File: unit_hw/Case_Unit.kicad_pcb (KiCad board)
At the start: 2 copper layers, 16.1 x 33.6 mm, 15 parts, among them J1 Conn_01x04, J3 RJ45, J4 Conn_01x03, U1 SPX3819M5-L-3-3, U2 STM32G030F6Px, U3 MAX487E

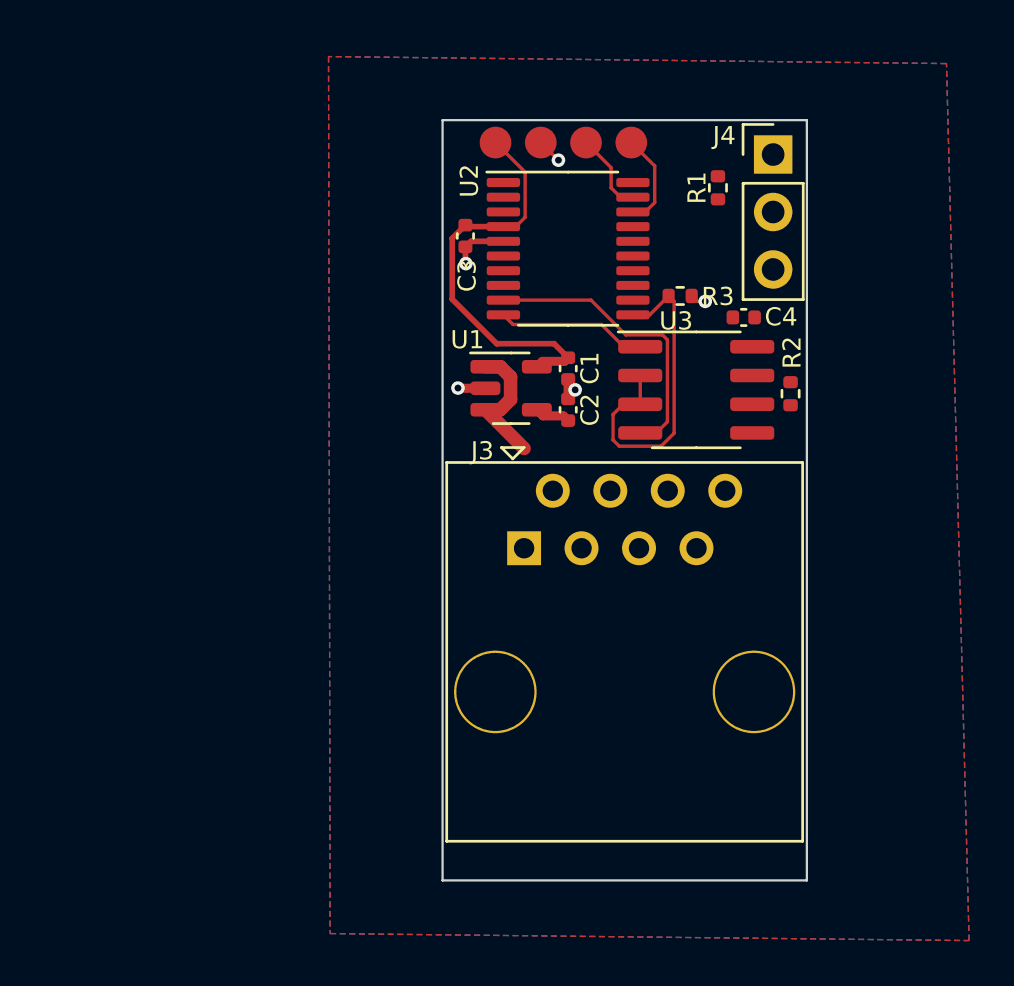
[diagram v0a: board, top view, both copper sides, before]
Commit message: Submit for fab (Rev. 2 unit)
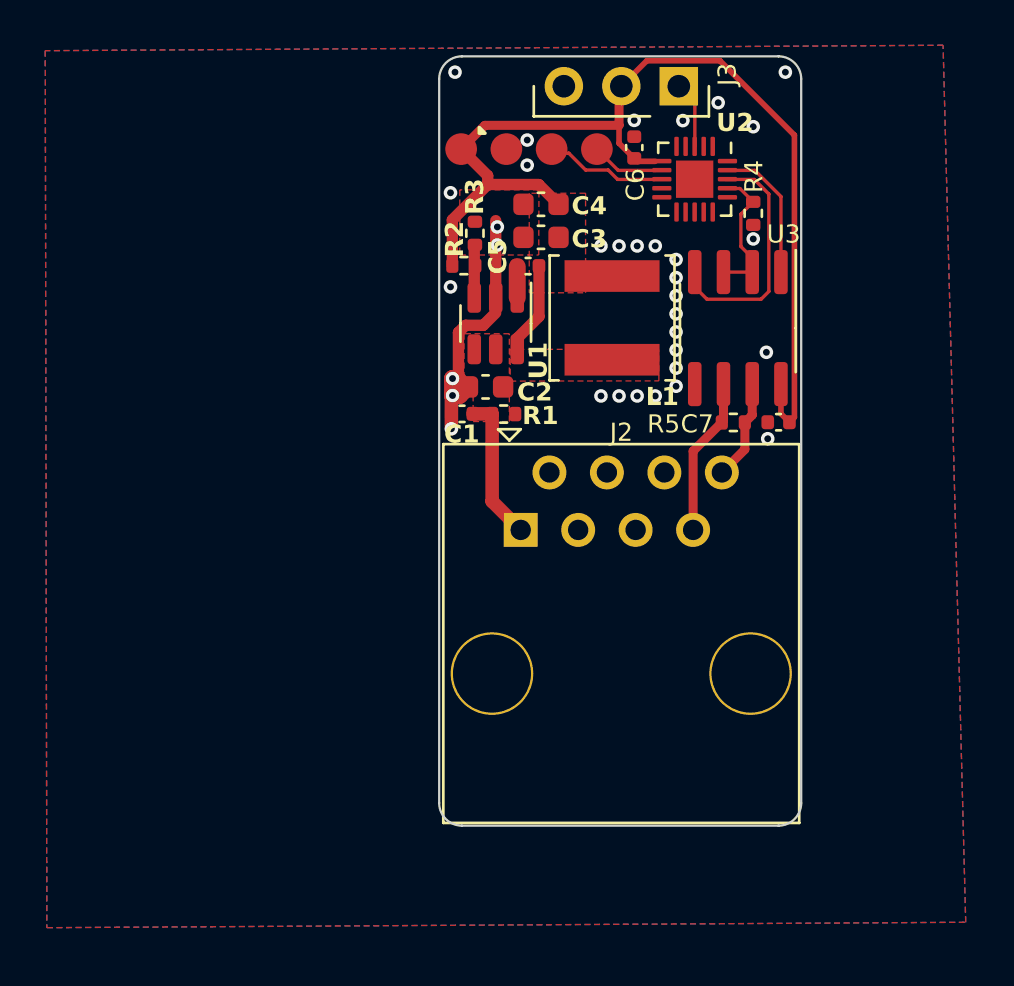
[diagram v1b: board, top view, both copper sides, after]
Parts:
- added C3: 22u, Capacitor_SMD:C_0603_1608Metric, F.Cu at (69.5, 40.0)
- added C4: 22u, Capacitor_SMD:C_0603_1608Metric, F.Cu at (69.5, 38.5)
- added C5: 100n, Capacitor_SMD:C_0402_1005Metric, F.Cu at (68.9, 41.3)
- added L1: 10u, Inductor_SMD:L_Changjiang_FNR5030S, F.Cu at (72.6, 43.6)
- added R2: 100k, Resistor_SMD:R_0402_1005Metric, F.Cu at (66.1, 41.2)
- added R3: 13k, Resistor_SMD:R_0402_1005Metric, F.Cu at (66.6, 39.8)
- C1: value 4.7u -> 100n
- C2: value 10n -> 22u; footprint Capacitor_SMD:C_0402_1005Metric -> Capacitor_SMD:C_0603_1608Metric
- R1: value 4.7k -> 1
- U1: value SPX3819M5-L-3-3 -> MT2492; footprint Package_TO_SOT_SMD:SOT-23-5 -> Package_TO_SOT_SMD:SOT-23-6
- U2: value STM32G030F6Px -> PY32F003F18U6; footprint Package_SO:TSSOP-20_4.4x6.5mm_P0.65mm -> Package_DFN_QFN:QFN-20-1EP_3x3mm_P0.4mm_EP1.65x1.65mm
- moved R1 13.8 mm to (67.8, 47.8), turned to 0 degrees
- moved C6 8.42 mm to (73.6, 36.0), turned to 90 degrees
- moved U2 6.38 mm to (76.3, 37.4), turned to -90 degrees
- moved J3 5.15 mm to (75.6, 33.3), turned to -90 degrees
- moved C1 5.10 mm to (66.0, 47.8), turned to 180 degrees
- moved C7 4.88 mm to (80.0, 48.2), turned to 180 degrees
- moved R4 4.87 mm to (78.9, 38.9), turned to -90 degrees
- moved C2 3.79 mm to (67.0, 46.6), turned to 180 degrees
- moved U3 3.29 mm to (78.2, 44.0), turned to -90 degrees
- moved U1 2.94 mm to (67.5, 43.8), turned to -90 degrees
- moved R5 2.83 mm to (78.0, 48.2), turned to 180 degrees
- moved J1 1.55 mm to (69.0, 36.1)
- moved J2 0.82 mm to (68.6, 52.9)
- moved G*** 0.53 mm to (70.8, 41.6)
- moved G*** 0.53 mm to (70.6, 36.6)
- renumbered C3 to C6, C4 to C7, J3 to J2, J4 to J3, R3 to R4, R2 to R5
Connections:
- C1 pad 1: +3V3 -> VIN
- C2 pad 1: Net-(U1-BP) -> Net-(U1-EN)
- C6 pad 1: +3V3 -> +5V
- J1 pad 1: +3V3 -> +5V
- J2 pad 1: +5V -> VIN
- J2 pad 3: unconnected-(J3-Pad3) -> GND
- J2 pad 4: unconnected-(J3-Pad4) -> GND
- J2 pad 5: unconnected-(J3-Pad5) -> GND
- J2 pad 6: unconnected-(J3-Pad6) -> GND
- R1 pad 1: +5V -> VIN
- R1 pad 2: /SERVO_OUT -> Net-(U1-EN)
- U1 pad 1: +5V -> Net-(U1-BS)
- U1 pad 3: +5V -> Net-(U1-FB)
- U1 pad 4: Net-(U1-BP) -> Net-(U1-EN)
- U1 pad 5: +3V3 -> Net-(U1-EN)
- U2 pad 10: /UART_RX -> unconnected-(U2-PB6-Pad10)
- U2 pad 11: /MAX487_DE -> unconnected-(U2-PB7-Pad11)
- U2 pad 14: /SERVO_OUT -> unconnected-(U2-PF1-Pad14)
- U2 pad 17: unconnected-(U2-PA12/PA10-Pad17) -> /MAX487_DE
- U2 pad 18: /SWDIO -> /UART_TX
- U2 pad 19: /SWCLK -> /UART_RX
- U2 pad 3: unconnected-(U2-PC15-Pad3) -> /SERVO_OUT
- U2 pad 4: +3V3 -> GND
- U2 pad 5: GND -> unconnected-(U2-PA12-Pad5)
- U2 pad 6: unconnected-(U2-NRST-Pad6) -> +5V
- U2 pad 7: unconnected-(U2-PA0-Pad7) -> /SWDIO
- U2 pad 8: unconnected-(U2-PA1-Pad8) -> /SWCLK
- U2 pad 9: /UART_TX -> unconnected-(U2-PB5-Pad9)
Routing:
- net +5V: track 6.01 -> 45.8 mm
- net +3V3: track 17.9 -> 0.00 mm
- net /MAX487_DE: track 14.9 -> 6.28 mm
- net /RS422+: track 0.00 -> 7.00 mm
- net VIN: track 0.00 -> 6.48 mm
- net GND: track 6.40 -> 11.7 mm, vias 5 -> 34
- net /RS422-: track 0.00 -> 4.46 mm
- net Net-(U1-SW): track 0.00 -> 4.08 mm
- net /SERVO_OUT: track 0.00 -> 2.79 mm
- net Net-(U1-FB): track 0.00 -> 2.35 mm
- net /UART_TX: track 13.0 -> 10.8 mm
- net Net-(U1-BP): track 1.58 -> 0.00 mm
- net /SWCLK: track 3.60 -> 5.14 mm
- net Net-(U1-BS): track 0.00 -> 1.38 mm
- net /SWDIO: track 4.21 -> 2.97 mm
- added copper zone on F.Cu, net +5V
- added copper zone on F.Cu, net Net-(U1-EN)
- added copper zone on F.Cu, net Net-(U1-SW)
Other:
- board size 16.1 x 33.6 mm -> 16 x 34 mm
- board text added: "Rev. 2"
- board text removed: "JLCJLCJLCJLC"
- board text removed: "Rev. 1"
